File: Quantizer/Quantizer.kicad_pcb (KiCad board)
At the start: 2 copper layers, 100 x 200 mm, 4 parts, among them J1 EuroPower

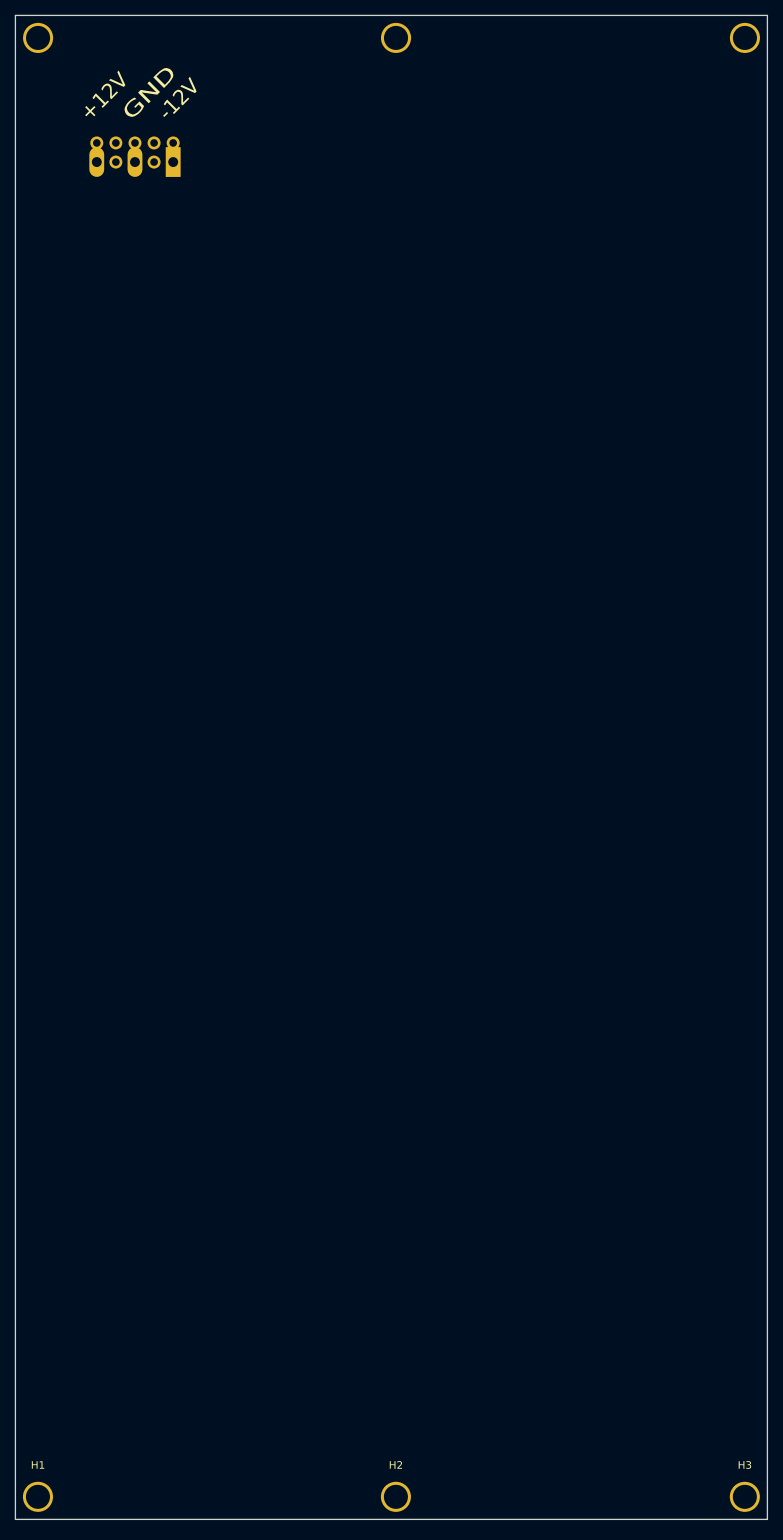
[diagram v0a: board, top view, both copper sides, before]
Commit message: Quantizer layout done!
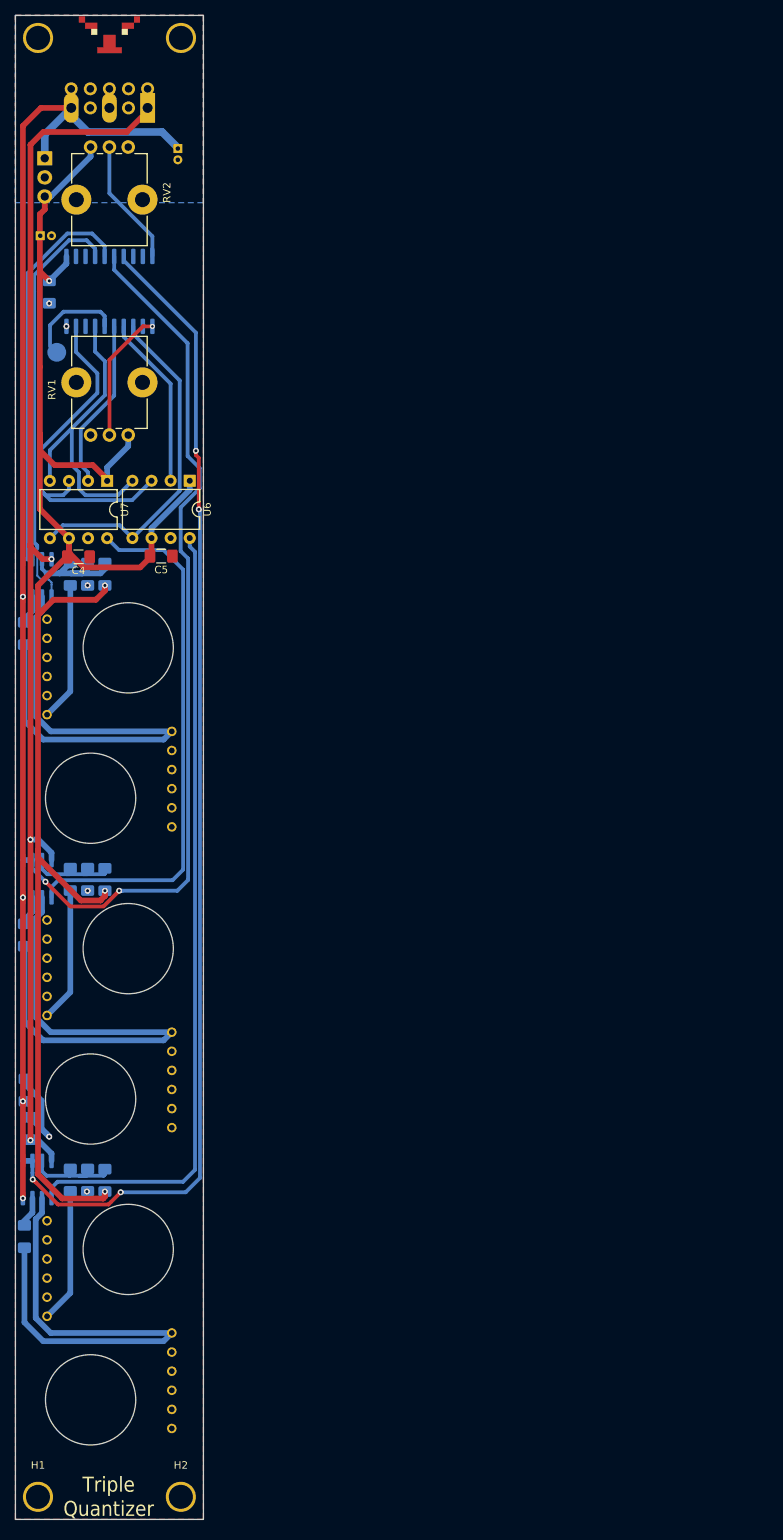
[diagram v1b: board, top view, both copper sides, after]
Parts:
- removed H3: Panel, Kosmo_panel:Kosmo_Panel_Dual_Mounting_Holes
- added C1: 10u, Capacitor_THT:CP_Radial_D4.0mm_P1.50mm, B.Cu at (33.7, 29.8)
- added C2: 1u, Capacitor_THT:CP_Radial_D4.0mm_P1.50mm, B.Cu at (15.4, 41.4)
- added C3: 100n, Capacitor_SMD:C_1206_3216Metric_Pad1.42x1.75mm_HandSolder, B.Cu at (16.6, 48.9)
- added C4: 100n, Capacitor_SMD:C_1206_3216Metric_Pad1.42x1.75mm_HandSolder, F.Cu at (20.5, 84.1)
- added C5: 100n, Capacitor_SMD:C_1206_3216Metric_Pad1.42x1.75mm_HandSolder, F.Cu at (31.5, 84.0)
- added C6: 100n, Capacitor_SMD:C_1206_3216Metric_Pad1.42x1.75mm_HandSolder, B.Cu at (13.4, 155.0)
- added C7: 100n, Capacitor_SMD:C_1206_3216Metric_Pad1.42x1.75mm_HandSolder, B.Cu at (14.0, 160.1)
- added D1: 1N4148, Diode_SMD:D_1206_3216Metric_Pad1.42x1.75mm_HandSolder, B.Cu at (24.0, 167.0)
- added D2: 1N4148, Diode_SMD:D_1206_3216Metric_Pad1.42x1.75mm_HandSolder, B.Cu at (21.7, 167.0)
- added D3: 1N4148, Diode_SMD:D_1206_3216Metric_Pad1.42x1.75mm_HandSolder, B.Cu at (24.0, 127.0)
- added D4: 1N4148, Diode_SMD:D_1206_3216Metric_Pad1.42x1.75mm_HandSolder, B.Cu at (21.7, 127.0)
- added D5: 1N4148, Diode_SMD:D_1206_3216Metric_Pad1.42x1.75mm_HandSolder, B.Cu at (24.0, 86.4)
- added D6: 1N4148, Diode_SMD:D_1206_3216Metric_Pad1.42x1.75mm_HandSolder, B.Cu at (21.7, 86.4)
- added J2: Prog, TestPoint:TestPoint_Pad_D2.5mm, B.Cu at (17.6, 56.9)
- added J3: IN1, telec:JackHole, F.Cu at (27.1, 176.2)
- added J4: IN2, telec:JackHole, F.Cu at (27.1, 136.2)
- added J5: IN3, telec:JackHole, F.Cu at (27.1, 96.2)
- added J6: OUT1, telec:JackHole, F.Cu at (22.1, 196.2)
- added J7: OUT2, telec:JackHole, F.Cu at (22.1, 156.2)
- added J8: OUT3, telec:JackHole, F.Cu at (22.1, 116.2)
- added LOGO1: telec, logo:telec-8, F.Cu at (24.6, 16.3)
- added R1: 100k, Resistor_SMD:R_1206_3216Metric_Pad1.42x1.75mm_HandSolder, B.Cu at (19.4, 167.0)
- added R2: 100k, Resistor_SMD:R_1206_3216Metric_Pad1.42x1.75mm_HandSolder, B.Cu at (19.4, 127.0)
- added R3: 100k, Resistor_SMD:R_1206_3216Metric_Pad1.42x1.75mm_HandSolder, B.Cu at (19.4, 86.4)
- added R4: 1k, Resistor_SMD:R_1206_3216Metric_Pad1.42x1.75mm_HandSolder, B.Cu at (13.3, 174.5)
- added R5: 1k, Resistor_SMD:R_1206_3216Metric_Pad1.42x1.75mm_HandSolder, B.Cu at (13.3, 134.4)
- added R6: 1k, Resistor_SMD:R_1206_3216Metric_Pad1.42x1.75mm_HandSolder, B.Cu at (13.3, 94.3)
- added RV1: 100k, Potentiometer_THT:Potentiometer_Alps_RK09K_Single_Vertical, F.Cu at (27.1, 67.9)
- added RV2: 100k, Potentiometer_THT:Potentiometer_Alps_RK09K_Single_Vertical, F.Cu at (22.1, 29.6)
- added U1: L7805, Package_TO_SOT_THT:TO-220-3_Vertical, B.Cu at (16.0, 31.1)
- added U2: TL082, Package_SO:SOIC-8_3.9x4.9mm_P1.27mm, B.Cu at (15.0, 166.9)
- added U3: TL082, Package_SO:SOIC-8_3.9x4.9mm_P1.27mm, B.Cu at (15.0, 126.9)
- added U4: TL082, Package_SO:SOIC-8_3.9x4.9mm_P1.27mm, B.Cu at (15.0, 86.9)
- added U5: ATtiny416-S, Package_SO:SOIC-20W_7.5x12.8mm_P1.27mm, B.Cu at (24.6, 48.8)
- added U6: MCP4801, Package_DIP:DIP-8_W7.62mm, F.Cu at (35.3, 74.0)
- added U7: MCP4801, Package_DIP:DIP-8_W7.62mm, F.Cu at (24.3, 74.0)
- H1, H2: value Panel -> Mounting_Holes
- moved H2 28.6 mm to (34.1, 209.1)
- moved J1 7.96 mm to (29.7, 24.4)
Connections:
- J1 pad 1: (no net) -> -12V
- J1 pad 2: (no net) -> GND
- J1 pad 3: (no net) -> +12V
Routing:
- net +5V: track 0.00 -> 232.0 mm, vias 0 -> 4
- net +12V: track 0.00 -> 177.8 mm, vias 0 -> 4
- net -12V: track 0.00 -> 165.5 mm, vias 0 -> 3
- net /IN1: track 0.00 -> 155.0 mm, vias 0 -> 4
- net /IN2: track 0.00 -> 115.7 mm, vias 0 -> 2
- net Net-(U2-Pad5): track 0.00 -> 105.7 mm
- net Net-(U3-Pad5): track 0.00 -> 71.6 mm
- net Net-(J8-PadT): track 0.00 -> 66.2 mm
- net Net-(J7-PadT): track 0.00 -> 66.2 mm
- net Net-(J6-PadT): track 0.00 -> 66.2 mm
- net /DAC0: track 0.00 -> 55.8 mm
- net /IN3: track 0.00 -> 53.8 mm
- net /SCK: track 0.00 -> 48.3 mm
- net /~LDAC: track 0.00 -> 45.7 mm
- net /MOSI: track 0.00 -> 40.8 mm
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- added copper zone on B.Cu, net GND
- added copper zone on F.Cu, net GND
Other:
- board size 100 x 200 mm -> 25 x 200 mm
- board text added: "Triple Quantizer"
